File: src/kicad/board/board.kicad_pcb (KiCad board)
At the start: 2 copper layers, 100.5 x 70.6 mm, 79 parts, among them J1 USB_C_Receptacle_USB2.0, J3 Micro_SD_Card_Det, J4 Conn_01x05_Male, J5 Conn_01x05_Male, J6 PWR_EN, J7 Screw_Terminal_Speaker, Q1 DMG2305UX, SW1 SW_Keyboard, SW2 SW_Keyboard, SW3 RotEncoder_S, SW4 SW_Keyboard, SW5 SW_Keyboard, SW6 BOOTSEL, U1 MCP23017_ML, U2 BQ25172, U3 TLV61070A, U4 XC6206P332MR, U5 MAX98357, U6 RP2040, U7 W25Q128JVS, Y1 X322512MSB4SI

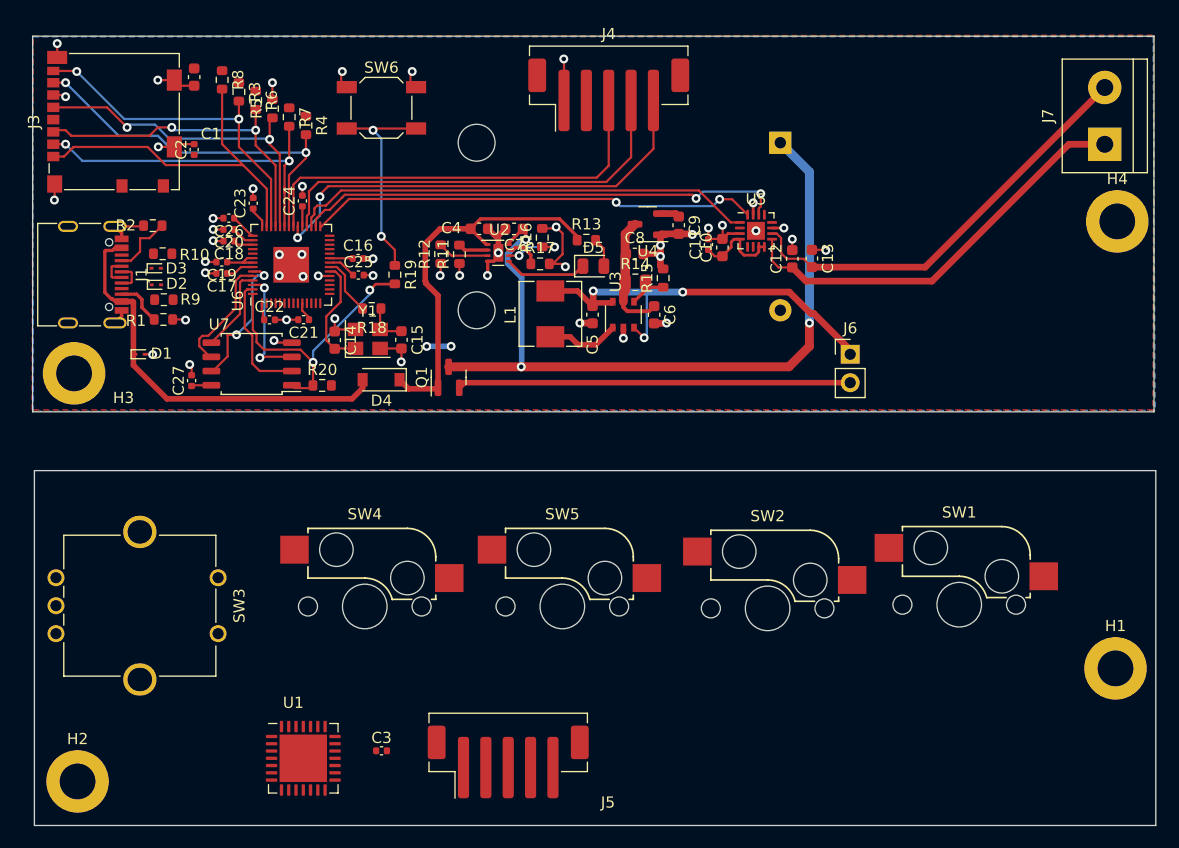
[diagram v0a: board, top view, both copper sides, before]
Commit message: update
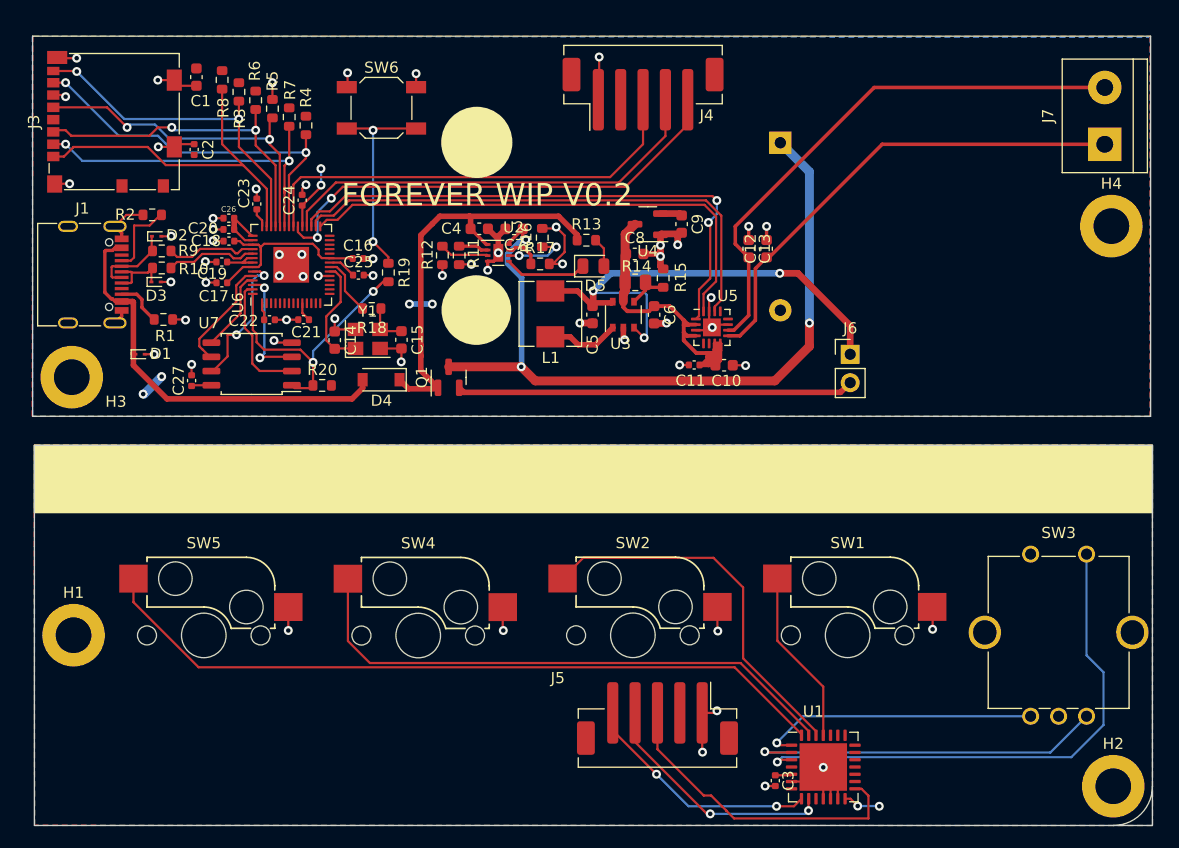
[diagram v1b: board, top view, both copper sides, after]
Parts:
- moved H1 93.2 mm to (101.2, 100.2)
- moved H2 92.6 mm to (194.2, 113.7)
- moved SW3 88.1 mm to (186.8, 107.4), turned to 90 degrees
- moved U1 46.5 mm to (168.3, 112.0)
- moved C3 35.3 mm to (164.0, 113.2), turned to -90 degrees
- moved SW5 32.2 mm to (112.9, 100.2)
- moved J5 13.9 mm to (153.4, 107.6), turned to 180 degrees
- moved SW2 12.3 mm to (151.2, 100.2)
- moved C11 10.8 mm to (156.7, 76.0), turned to 180 degrees
- moved C10 10.5 mm to (159.4, 76.0), turned to 0 degrees
- moved SW1 10.3 mm to (170.4, 100.2)
- moved U5 9.50 mm to (158.3, 72.6)
- moved C13 5.72 mm to (161.6, 65.6)
- moved SW4 5.44 mm to (132.0, 100.2)
- moved R9 4.36 mm to (109.1, 65.8)
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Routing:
- net B3: track 0.00 -> 66.8 mm
- net B2: track 0.00 -> 50.5 mm
- net B6: track 0.00 -> 47.8 mm, vias 0 -> 1
- net B1: track 0.00 -> 33.9 mm
- net B5: track 0.00 -> 32.6 mm, vias 0 -> 1
- net /Input/INT: track 0.00 -> 28.2 mm
- net /Input/GND_LOCAL: track 0.00 -> 26.9 mm, vias 0 -> 8
- net B4: track 0.00 -> 25.1 mm, vias 0 -> 1
- net /Input/SDA: track 0.00 -> 22.0 mm, vias 0 -> 2
- net /Input/SCK: track 0.00 -> 21.5 mm, vias 0 -> 2
- net VDD: track 26.5 -> 47.3 mm
- net B0: track 0.00 -> 15.7 mm
- net +1V1: track 6.46 -> 17.5 mm
- net Net-(C13-Pad2): track 38.5 -> 49.1 mm
- net /USB_D-: track 0.00 -> 8.17 mm
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- added copper zone on F.Cu, net /Input/3.3V_LOCAL
- added copper zone on B.Cu, net /Input/GND_LOCAL
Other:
- board size 100.5 x 70.6 mm -> 100.2 x 70.6 mm
- board text added: "FOREVER WIP V0.2"
